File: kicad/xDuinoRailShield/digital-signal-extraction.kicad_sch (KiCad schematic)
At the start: 11 parts, among them Q1 T2N7002BK, U301 6N137, U302 EL817

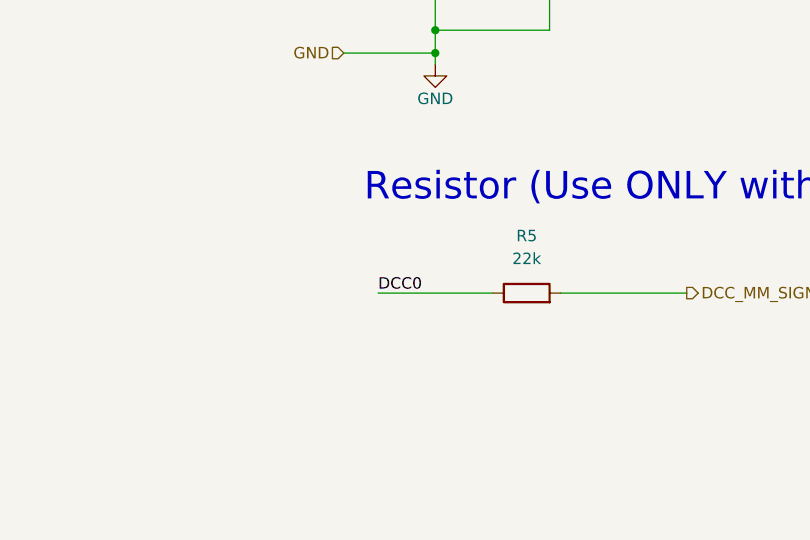
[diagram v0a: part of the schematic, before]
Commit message: Final version
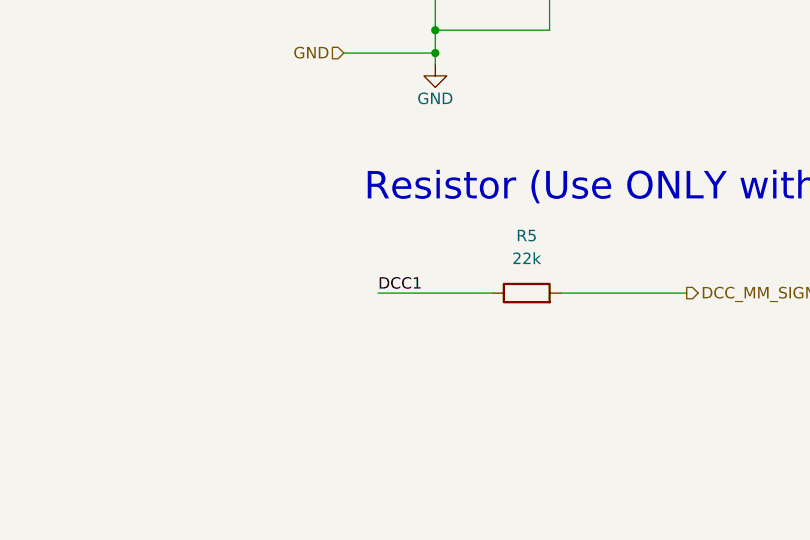
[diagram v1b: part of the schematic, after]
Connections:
- net DCC0: no longer R5.1
- net DCC1: now also R5.1
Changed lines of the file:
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@@
 		)
 	)
-	(label "DCC0"
+	(label "DCC1"
 		(at 154.94 110.49 0)
 		(fields_autoplaced yes)

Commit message: Refactoring & Sound
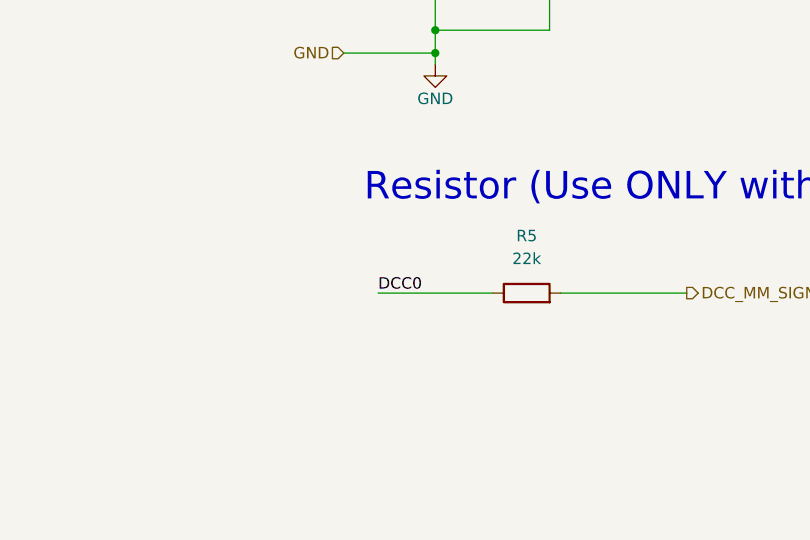
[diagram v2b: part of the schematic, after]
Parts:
- R5: footprint Resistor_SMD:R_0805_2012Metric_Pad1.20x1.40mm_HandSolder -> Resistor_SMD:R_0402_1005Metric_Pad0.72x0.64mm_HandSolder
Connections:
- net DCC0: now also R5.1
- net DCC1: no longer R5.1
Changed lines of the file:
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@@
 		)
 	)
-	(label "DCC1"
+	(label "DCC0"
 		(at 154.94 110.49 0)
 		(fields_autoplaced yes)
@@
 			)
 		)
-		(property "Footprint" "Resistor_SMD:R_0805_2012Metric_Pad1.20x1.40mm_HandSolder"
+		(property "Footprint" "Resistor_SMD:R_0402_1005Metric_Pad0.72x0.64mm_HandSolder"
 			(at 171.45 112.268 90)
 			(effects
